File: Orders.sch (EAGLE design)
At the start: 18 parts, among them J1 10104111-0001LF

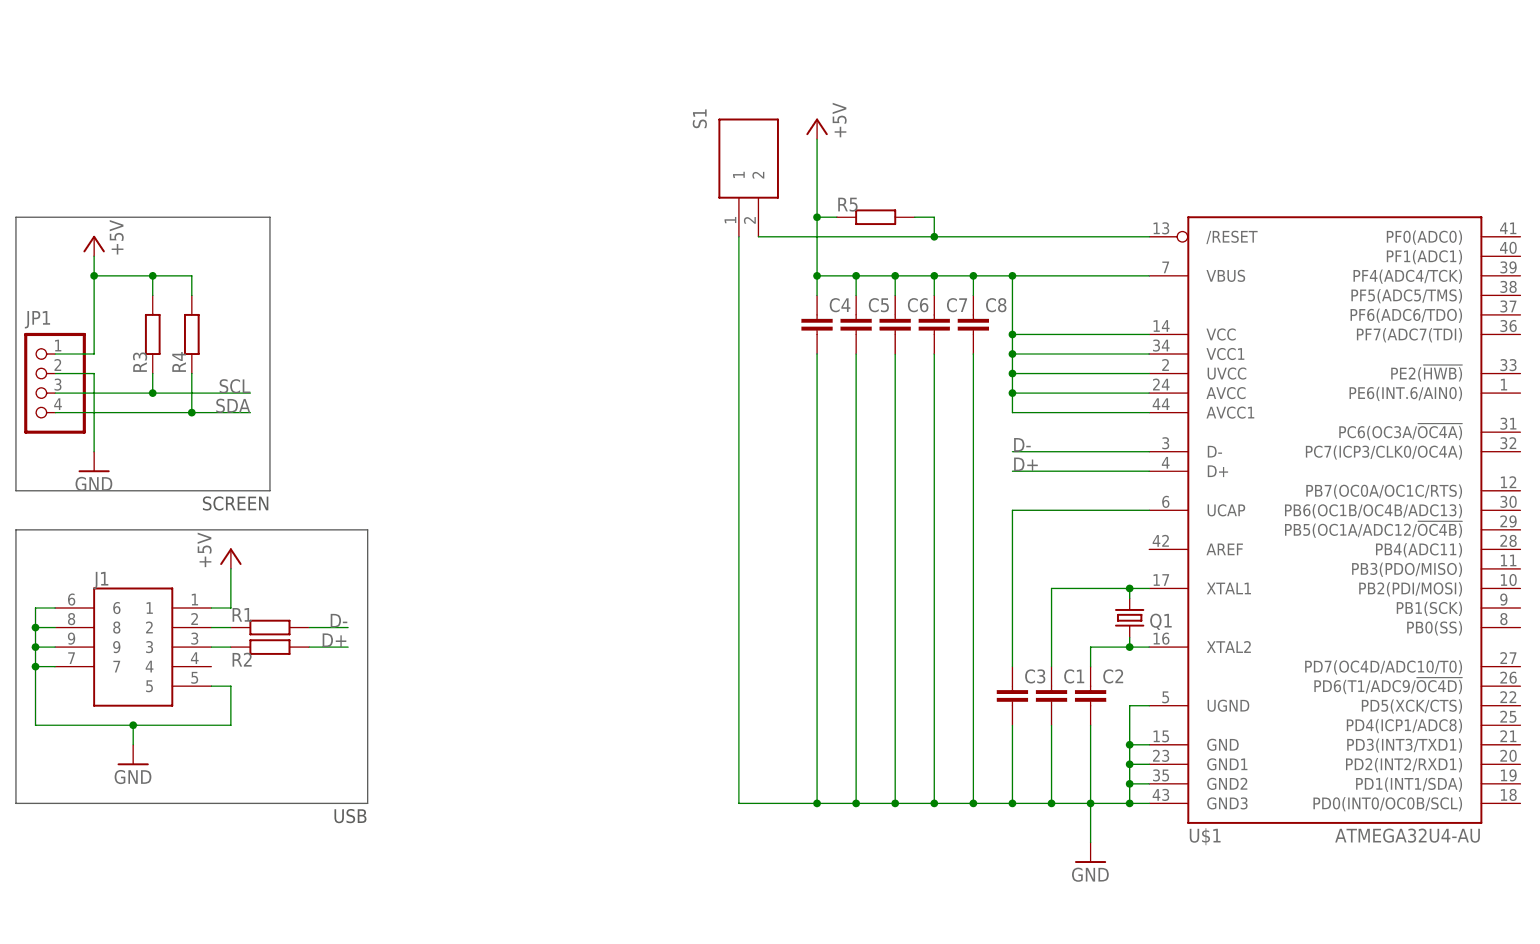
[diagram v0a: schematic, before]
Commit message: Finished schematic
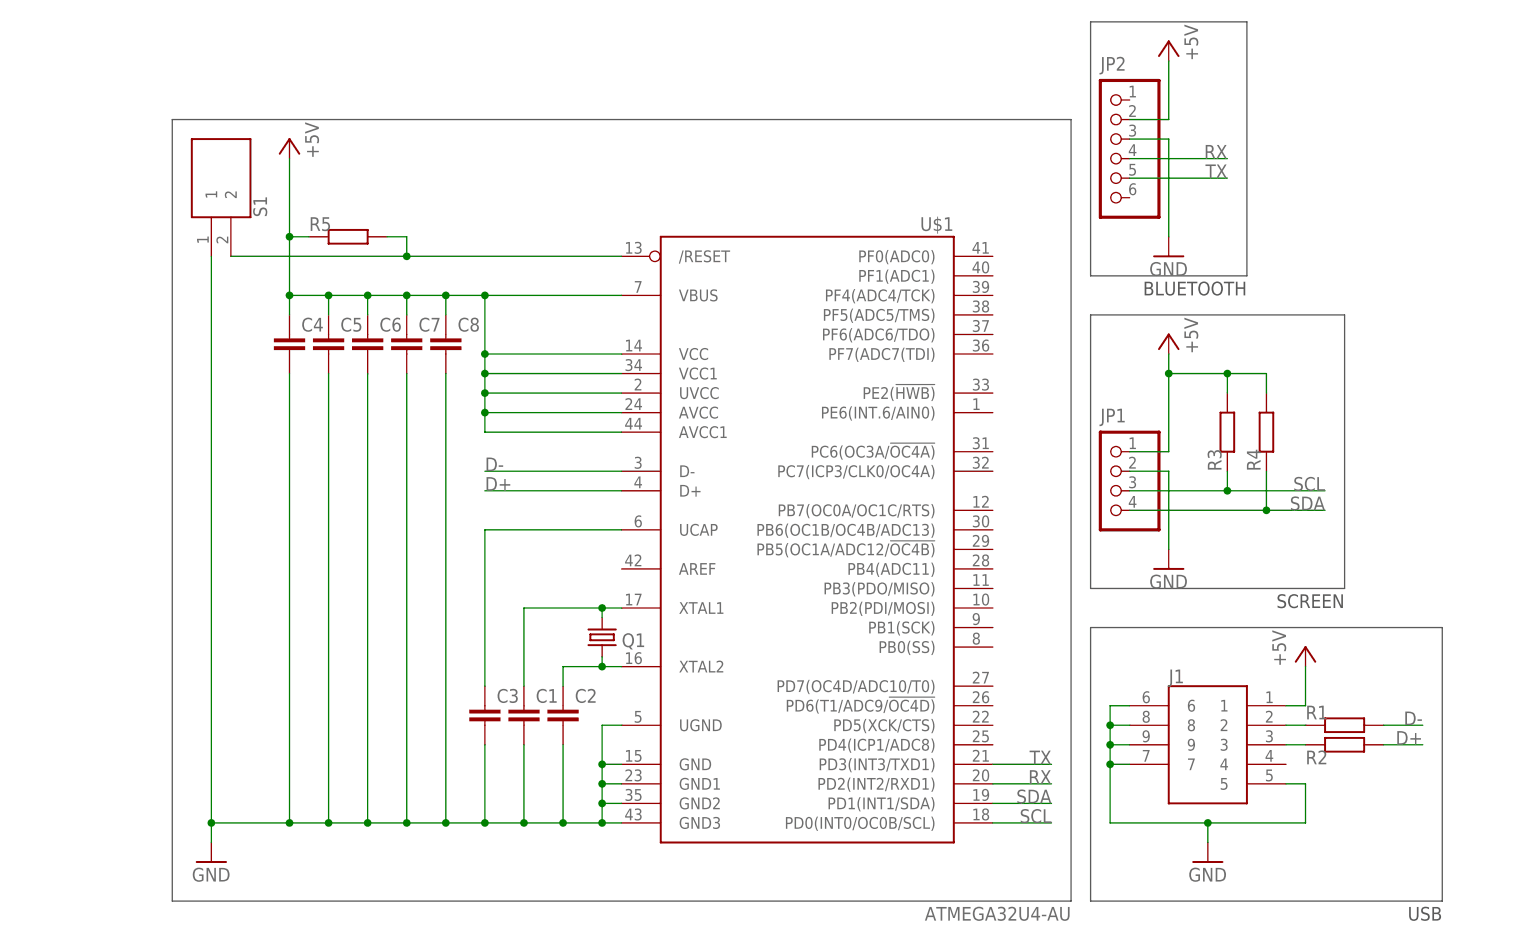
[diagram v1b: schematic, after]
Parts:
- added JP2: (no value), pinhead:PINHD-1X6
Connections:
- new net RX: JP2.4, U$1.PD2(INT2/RXD1)
- new net TX: JP2.5, U$1.PD3(INT3/TXD1)
- net +5V: now also JP2.2
- net GND: now also JP2.3
- net SCL: now also U$1.PD0(INT0/OC0B/SCL)
- net SDA: now also U$1.PD1(INT1/SDA)
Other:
- note added: "BLUETOOTH"
- moved on the sheet: C1, C2, C3, C4, C5, C6, C7, C8, J1, JP1, Q1, R1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
